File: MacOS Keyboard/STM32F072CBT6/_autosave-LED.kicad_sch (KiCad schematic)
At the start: 210 parts

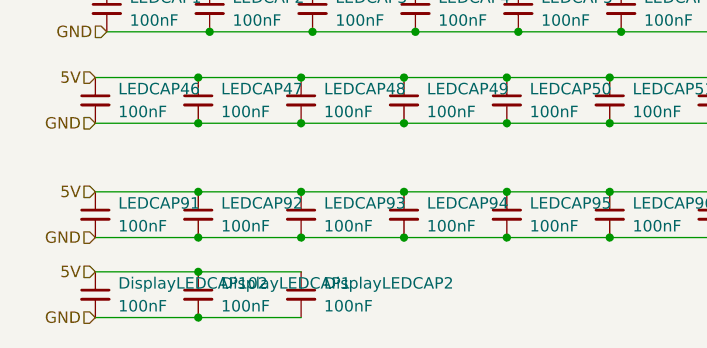
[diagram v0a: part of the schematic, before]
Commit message: changes
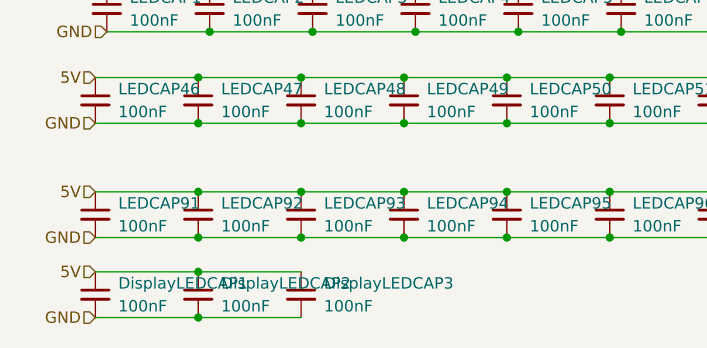
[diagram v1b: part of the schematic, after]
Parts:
- renumbered DisplayLEDCAP102 to DisplayLEDCAP1, DisplayLEDCAP1 to DisplayLEDCAP2, DisplayLEDCAP2 to DisplayLEDCAP3
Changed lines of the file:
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@@
 		(dnp no)
 		(fields_autoplaced yes)
-		(property "Reference" "DisplayLEDCAP1"
+		(property "Reference" "DisplayLEDCAP2"
 			(at 34.29 210.8262 0)
 			(effects
@@
 			(project "ScottoModules"
 				(path "/92054fa3-5ad0-458e-bd73-acbcf8d11243/e384a74f-66b6-47af-af7a-2f4cea2d8317"
-					(reference "DisplayLEDCAP1")
+					(reference "DisplayLEDCAP2")
 					(unit 1)
 				)
@@
 		(dnp no)
 		(fields_autoplaced yes)
-		(property "Reference" "DisplayLEDCAP2"
+		(property "Reference" "DisplayLEDCAP3"
 			(at 45.72 210.8262 0)
 			(effects
@@
 			(project "ScottoModules"
 				(path "/92054fa3-5ad0-458e-bd73-acbcf8d11243/e384a74f-66b6-47af-af7a-2f4cea2d8317"
-					(reference "DisplayLEDCAP2")
+					(reference "DisplayLEDCAP3")
 					(unit 1)
 				)
@@
 		(dnp no)
 		(fields_autoplaced yes)
-		(property "Reference" "DisplayLEDCAP102"
+		(property "Reference" "DisplayLEDCAP1"
 			(at 22.86 210.8262 0)
 			(effects
@@
 			(project "ScottoModules"
 				(path "/92054fa3-5ad0-458e-bd73-acbcf8d11243/e384a74f-66b6-47af-af7a-2f4cea2d8317"
-					(reference "DisplayLEDCAP102")
+					(reference "DisplayLEDCAP1")
 					(unit 1)
 				)
